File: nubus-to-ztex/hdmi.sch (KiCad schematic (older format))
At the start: 10 parts, among them J5 10029449-111RLF (HDMI A), U9 TPD12S016PWR

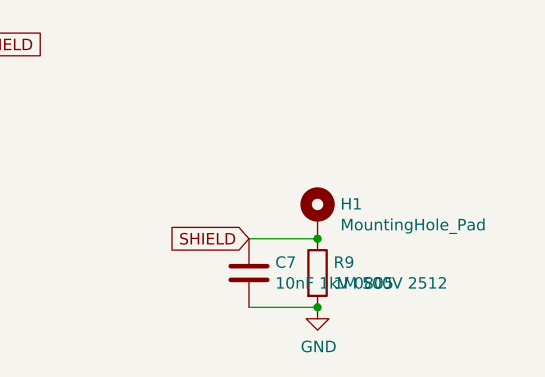
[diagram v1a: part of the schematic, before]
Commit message: some BoM optimization
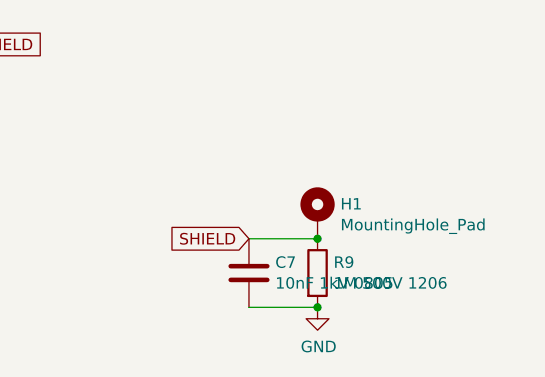
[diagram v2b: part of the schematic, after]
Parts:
- C20: MPN CC0603KRX7R8BB103 -> 0603B103K500NT; URL https://www.lcsc.com/product-detail/Multilayer-Ceramic-Capacitors-MLCC-SMD-SMT_YAGEO-CC0603KRX7R8BB103_C327204.html -> https://www.lcsc.com/product-detail/Multilayer-Ceramic-Capacitors-MLCC-SMD-SMT_FH-Guangdong-Fenghua-Advanced-Tech-0603B103K500NT_C57112.html
- C22, C23, C24: MPN CC0603KRX7R8BB104 -> CC0603KRX7R9BB104; URL https://www.lcsc.com/product-detail/Multilayer-Ceramic-Capacitors-MLCC-SMD-SMT_YAGEO-CC0603KRX7R8BB104_C92490.html -> https://www.lcsc.com/product-detail/Multilayer-Ceramic-Capacitors-MLCC-SMD-SMT_YAGEO-CC0603KRX7R9BB104_C14663.html
- C7: MPN C0805V103KCRACTU -> C0805X103K501T; MPN-ALT (none) -> C0805V103KCRACTU; MPN-ALT2 (none) -> TCC0805X7R103K501FT; URL https://www.lcsc.com/product-detail/Multilayer-Ceramic-Capacitors-MLCC-SMD-SMT_KEMET-C0805V103KCRACTU_C2170011.html -> https://www.lcsc.com/product-detail/Multilayer-Ceramic-Capacitors-MLCC-SMD-SMT_IHHEC-HOLY-STONE-ENTERPRISE-CO-LTD-C0805X103K501T_C105950.html; URL-ALT (none) -> https://www.lcsc.com/product-detail/Multilayer-Ceramic-Capa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; URL-ALT2 (none) -> https://www.lcsc.com/product-detail/Multilayer-Ceramic-Capa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
- R9: value 1M 500V 2512 -> 1M 500V 1206; footprint Resistor_SMD:R_2512_6332Metric -> Resistor_SMD:R_1206_3216Metric; MPN AS25J1004ET -> HR1206J1M00P05Z; MPN-ALT (none) -> KTR18EZPF1004; URL https://www.lcsc.com/product-detail/Chip-Resistor-Surface-Mount_Ohmite-AS25J1004ET_C2546765.html -> https://www.lcsc.com/product-detail/Chip-Resistor-Surface-Mount_Ever-Ohms-Tech-HR1206J1M00P05Z_C175518.html; URL-ALT (none) -> https://www.lcsc.com/product-detail/Chip-Resistor-Surface-M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
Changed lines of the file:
@@
 F 3 "" H 7300 1700 50  0000 C CNN
 F 4 "www.yageo.com" H 7300 1700 50  0001 C CNN "MNF1_URL"
-F 5 "CC0603KRX7R8BB104" H 7300 1700 50  0001 C CNN "MPN"
+F 5 "CC0603KRX7R9BB104" H 7300 1700 50  0001 C CNN "MPN"
 F 6 "603-CC603KRX7R8BB104" H 7300 1700 50  0001 C CNN "Mouser"
 F 7 "?" H 7300 1700 50  0001 C CNN "Digikey"
@@
 F 9 "?" H 7300 1700 50  0001 C CNN "Koncar"
 F 10 "TB" H 7300 1700 50  0001 C CNN "Side"
-F 11 "https://www.lcsc.com/product-detail/Multilayer-Ceramic-Capacitors-MLCC-SMD-SMT_YAGEO-CC0603KRX7R8BB104_C92490.html" H 3000 6050 50  0001 C CNN "URL"
+F 11 "https://www.lcsc.com/product-detail/Multilayer-Ceramic-Capacitors-MLCC-SMD-SMT_YAGEO-CC0603KRX7R9BB104_C14663.html" H 3000 6050 50  0001 C CNN "URL"
 	1    7300 1700
 	1    0    0    -1
@@
 F 3 "" H 2250 1600 50  0000 C CNN
 F 4 "www.yageo.com" H 2250 1600 50  0001 C CNN "MNF1_URL"
-F 5 "CC0603KRX7R8BB104" H 2250 1600 50  0001 C CNN "MPN"
+F 5 "CC0603KRX7R9BB104" H 2250 1600 50  0001 C CNN "MPN"
 F 6 "603-CC603KRX7R8BB104" H 2250 1600 50  0001 C CNN "Mouser"
 F 7 "?" H 2250 1600 50  0001 C CNN "Digikey"
@@
 F 9 "?" H 2250 1600 50  0001 C CNN "Koncar"
 F 10 "TB" H 2250 1600 50  0001 C CNN "Side"
-F 11 "https://www.lcsc.com/product-detail/Multilayer-Ceramic-Capacitors-MLCC-SMD-SMT_YAGEO-CC0603KRX7R8BB104_C92490.html" H 2250 1600 50  0001 C CNN "URL"
+F 11 "https://www.lcsc.com/product-detail/Multilayer-Ceramic-Capacitors-MLCC-SMD-SMT_YAGEO-CC0603KRX7R9BB104_C14663.html" H 2250 1600 50  0001 C CNN "URL"
 	1    2250 1600
 	0    1    1    0
@@
 F 3 "" H 2450 1900 50  0000 C CNN
 F 4 "www.yageo.com" H 2450 1900 50  0001 C CNN "MNF1_URL"
-F 5 "CC0603KRX7R8BB104" H 2450 1900 50  0001 C CNN "MPN"
+F 5 "CC0603KRX7R9BB104" H 2450 1900 50  0001 C CNN "MPN"
 F 6 "603-CC603KRX7R8BB104" H 2450 1900 50  0001 C CNN "Mouser"
 F 7 "?" H 2450 1900 50  0001 C CNN "Digikey"
@@
 F 9 "?" H 2450 1900 50  0001 C CNN "Koncar"
 F 10 "TB" H 2450 1900 50  0001 C CNN "Side"
-F 11 "https://www.lcsc.com/product-detail/Multilayer-Ceramic-Capacitors-MLCC-SMD-SMT_YAGEO-CC0603KRX7R8BB104_C92490.html" H 3000 6050 50  0001 C CNN "URL"
+F 11 "https://www.lcsc.com/product-detail/Multilayer-Ceramic-Capacitors-MLCC-SMD-SMT_YAGEO-CC0603KRX7R9BB104_C14663.html" H 3000 6050 50  0001 C CNN "URL"
 	1    2450 1900
 	0    1    1    0
@@
 F 3 "" H 2250 1100 50  0000 C CNN
 F 4 "www.yageo.com" H 2250 1100 50  0001 C CNN "MNF1_URL"
-F 5 "CC0603KRX7R8BB103" H 2250 1100 50  0001 C CNN "MPN"
+F 5 "0603B103K500NT" H 2250 1100 50  0001 C CNN "MPN"
 F 6 "603-CC603KRX7R8BB103" H 2250 1100 50  0001 C CNN "Mouser"
-F 7 "https://www.lcsc.com/product-detail/Multilayer-Ceramic-Capacitors-MLCC-SMD-SMT_YAGEO-CC0603KRX7R8BB103_C327204.html" H 2250 1100 50  0001 C CNN "URL"
+F 7 "https://www.lcsc.com/product-detail/Multilayer-Ceramic-Capacitors-MLCC-SMD-SMT_FH-Guangdong-Fenghua-Advanced-Tech-0603B103K500NT_C57112.html" H 2250 1100 50  0001 C CNN "URL"
 	1    2250 1100
 	0    1    1    0
@@
 F 2 "Capacitor_SMD:C_0805_2012Metric" H 8238 4500 50  0001 C CNN
 F 3 "~" H 8200 4650 50  0001 C CNN
-F 4 "C0805V103KCRACTU" H 8200 4650 50  0001 C CNN "MPN"
-F 5 "https://www.lcsc.com/product-detail/Multilayer-Ceramic-Capacitors-MLCC-SMD-SMT_KEMET-C0805V103KCRACTU_C2170011.html" H 8200 4650 50  0001 C CNN "URL"
+F 4 "C0805V103KCRACTU" H 8200 4650 50  0001 C CNN "MPN-ALT"
+F 5 "https://www.lcsc.com/product-detail/Multilayer-Ceramic-Capacitors-MLCC-SMD-SMT_KEMET-C0805V103KCRACTU_C2170011.html" H 8200 4650 50  0001 C CNN "URL-ALT"
+F 6 "TCC0805X7R103K501FT" H 8200 4650 50  0001 C CNN "MPN-ALT2"
+F 7 "https://www.lcsc.com/product-detail/Multilayer-Ceramic-Capacitors-MLCC-SMD-SMT_CCTC-TCC0805X7R103K501FT_C282729.html" H 8200 4650 50  0001 C CNN "URL-ALT2"
+F 8 "C0805X103K501T" H 8200 4650 50  0001 C CNN "MPN"
+F 9 "https://www.lcsc.com/product-detail/Multilayer-Ceramic-Capacitors-MLCC-SMD-SMT_IHHEC-HOLY-STONE-ENTERPRISE-CO-LTD-C0805X103K501T_C105950.html" H 8200 4650 50  0001 C CNN "URL"
 	1    8200 4650
 	1    0    0    -1
@@
 AR Path="/61B62C00/641A2763" Ref="R9"  Part="1"
 F 0 "R9" H 8570 4696 50  0000 L CNN
-F 1 "1M 500V 2512" H 8570 4605 50  0000 L CNN
-F 2 "Resistor_SMD:R_2512_6332Metric" V 8430 4650 50  0001 C CNN
+F 1 "1M 500V 1206" H 8570 4605 50  0000 L CNN
+F 2 "Resistor_SMD:R_1206_3216Metric" V 8430 4650 50  0001 C CNN
 F 3 "~" H 8500 4650 50  0001 C CNN
-F 4 "AS25J1004ET" H 8500 4650 50  0001 C CNN "MPN"
-F 5 "https://www.lcsc.com/product-detail/Chip-Resistor-Surface-Mount_Ohmite-AS25J1004ET_C2546765.html" H 8500 4650 50  0001 C CNN "URL"
+F 4 "HR1206J1M00P05Z" H 8500 4650 50  0001 C CNN "MPN"
+F 5 "https://www.lcsc.com/product-detail/Chip-Resistor-Surface-Mount_Ever-Ohms-Tech-HR1206J1M00P05Z_C175518.html" H 8500 4650 50  0001 C CNN "URL"
+F 6 "KTR18EZPF1004" H 8500 4650 50  0001 C CNN "MPN-ALT"
+F 7 "https://www.lcsc.com/product-detail/Chip-Resistor-Surface-Mount_ROHM-Semicon-KTR18EZPF1004_C253347.html" H 8500 4650 50  0001 C CNN "URL-ALT"
 	1    8500 4650
 	1    0    0    -1
